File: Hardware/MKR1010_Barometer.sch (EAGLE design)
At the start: 2 parts

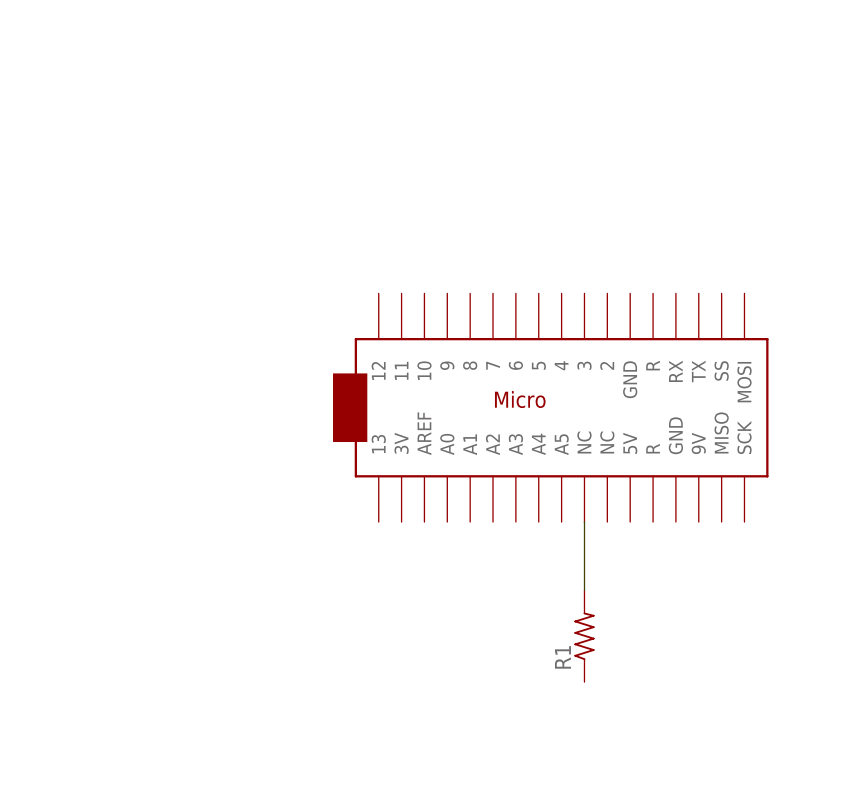
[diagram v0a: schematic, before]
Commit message: schematic capture
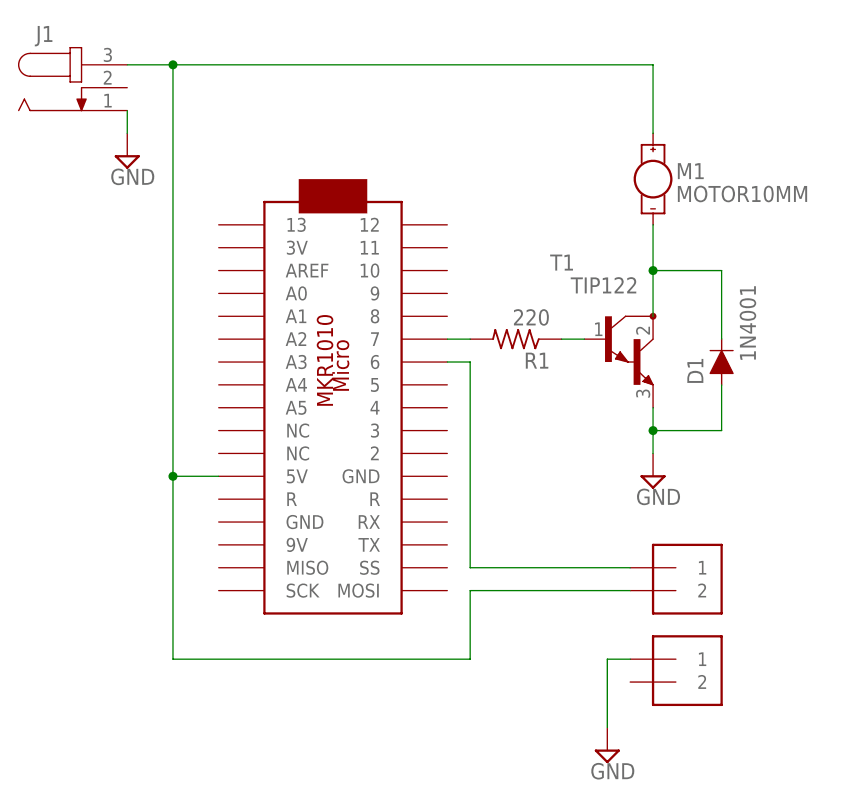
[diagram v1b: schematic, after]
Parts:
- removed U$1: ARDUINOMICRO, adafruit:ARDUINOMICRO
- added D1: 1N4001, SparkFun-DiscreteSemi:DIODE-PTH
- added J1: (no value), con-jack:JACK-PLUG0
- added J2, J3: 1X2-3.5MM, adafruit:1X2-3.5MM
- added M1: MOTOR10MM, SparkFun-Electromechanical:MOTOR10MM
- added MKR1010: ARDUINOMICRO, adafruit:ARDUINOMICRO
- added T1: TIP122, transistor:TIP122
- R1: value (none) -> 220
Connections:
- new net GND: D1.A, J1.1, J3.1, T1.E
- new net N$2: R1.1, T1.B
- new net N$3: D1.C, M1.-, T1.C
- new net N$4: J1.3, J2.2, M1.+, MKR1010.5V
- new net N$5: J2.1, MKR1010.6
- net N$1: now also MKR1010.7; no longer U$1.NC@2
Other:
- note added: "MKR1010"
- moved on the sheet: R1
